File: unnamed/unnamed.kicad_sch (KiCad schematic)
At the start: 70 parts, among them J1 Serial, J2 Serial, SW1 SW_Push, SW10 SW_Push, SW11 SW_Push, SW12 SW_Push, SW13 SW_Push, SW14 SW_Push, SW15 SW_Push, SW16 SW_Push, SW17 SW_Push, SW18 SW_Push, SW19 SW_Push, SW2 SW_Push, SW20 SW_Push, SW21 SW_Push, SW22 SW_Push, SW23 SW_Push, SW24 SW_Push, SW25 SW_SPST, SW26 SW_SPST, SW3 SW_Push, SW4 SW_Push, SW5 SW_Push, SW6 SW_Push, SW7 SW_Push, SW8 SW_Push, SW9 SW_Push, U1 eliteC, U2 eliteC

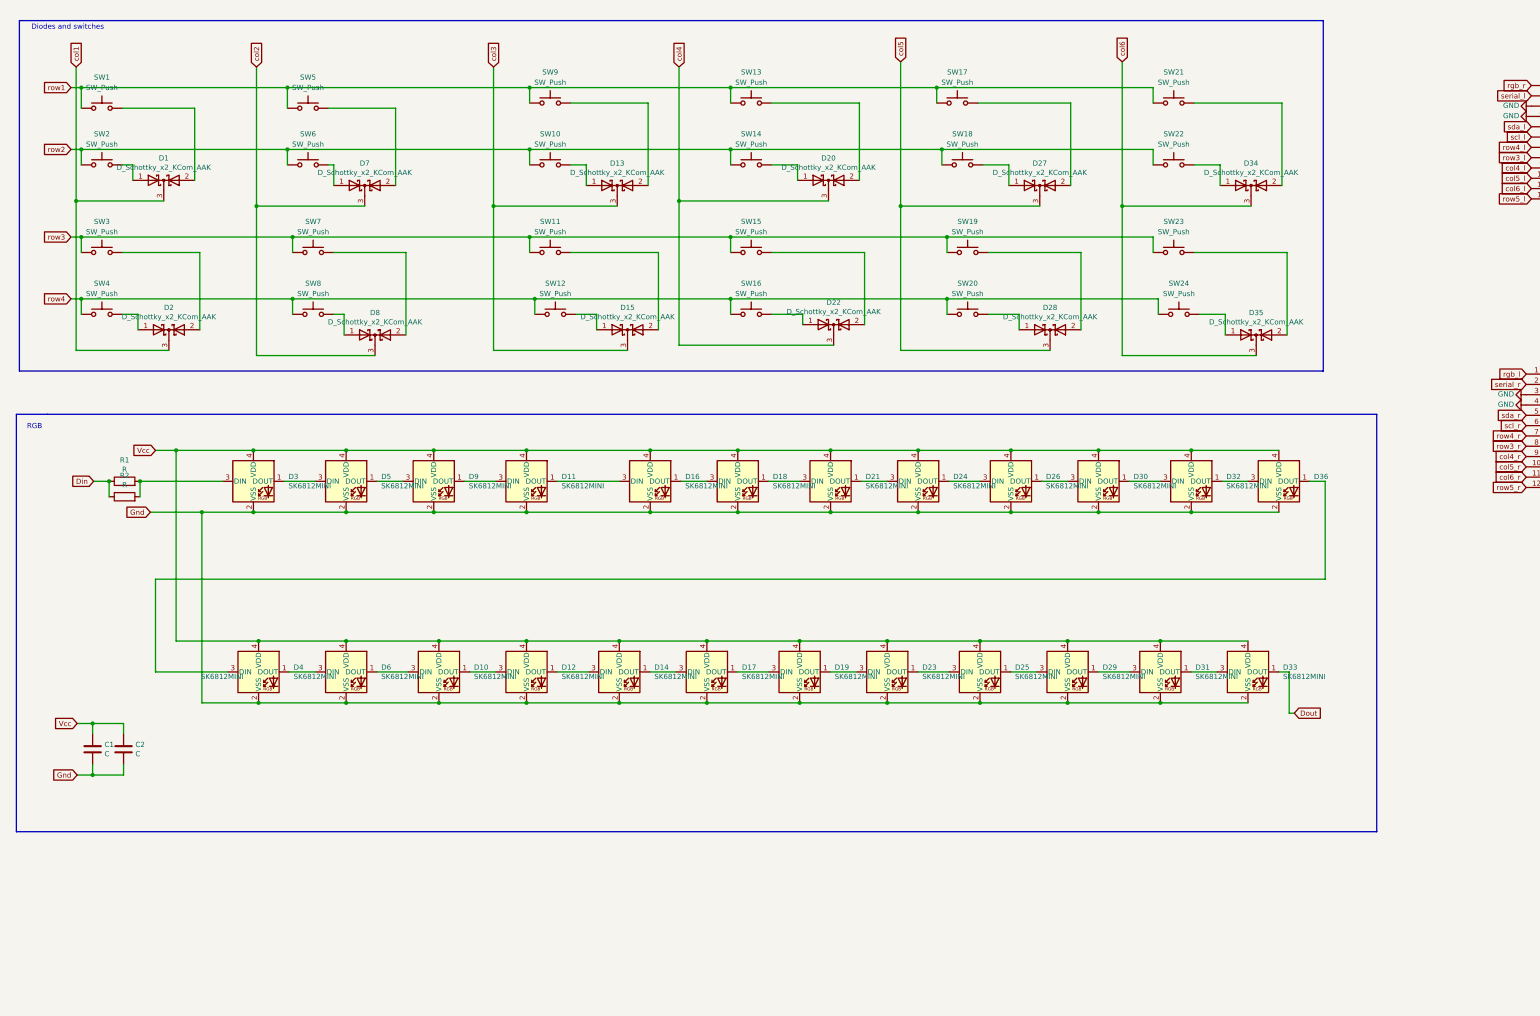
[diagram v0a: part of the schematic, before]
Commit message: go back to 3x5
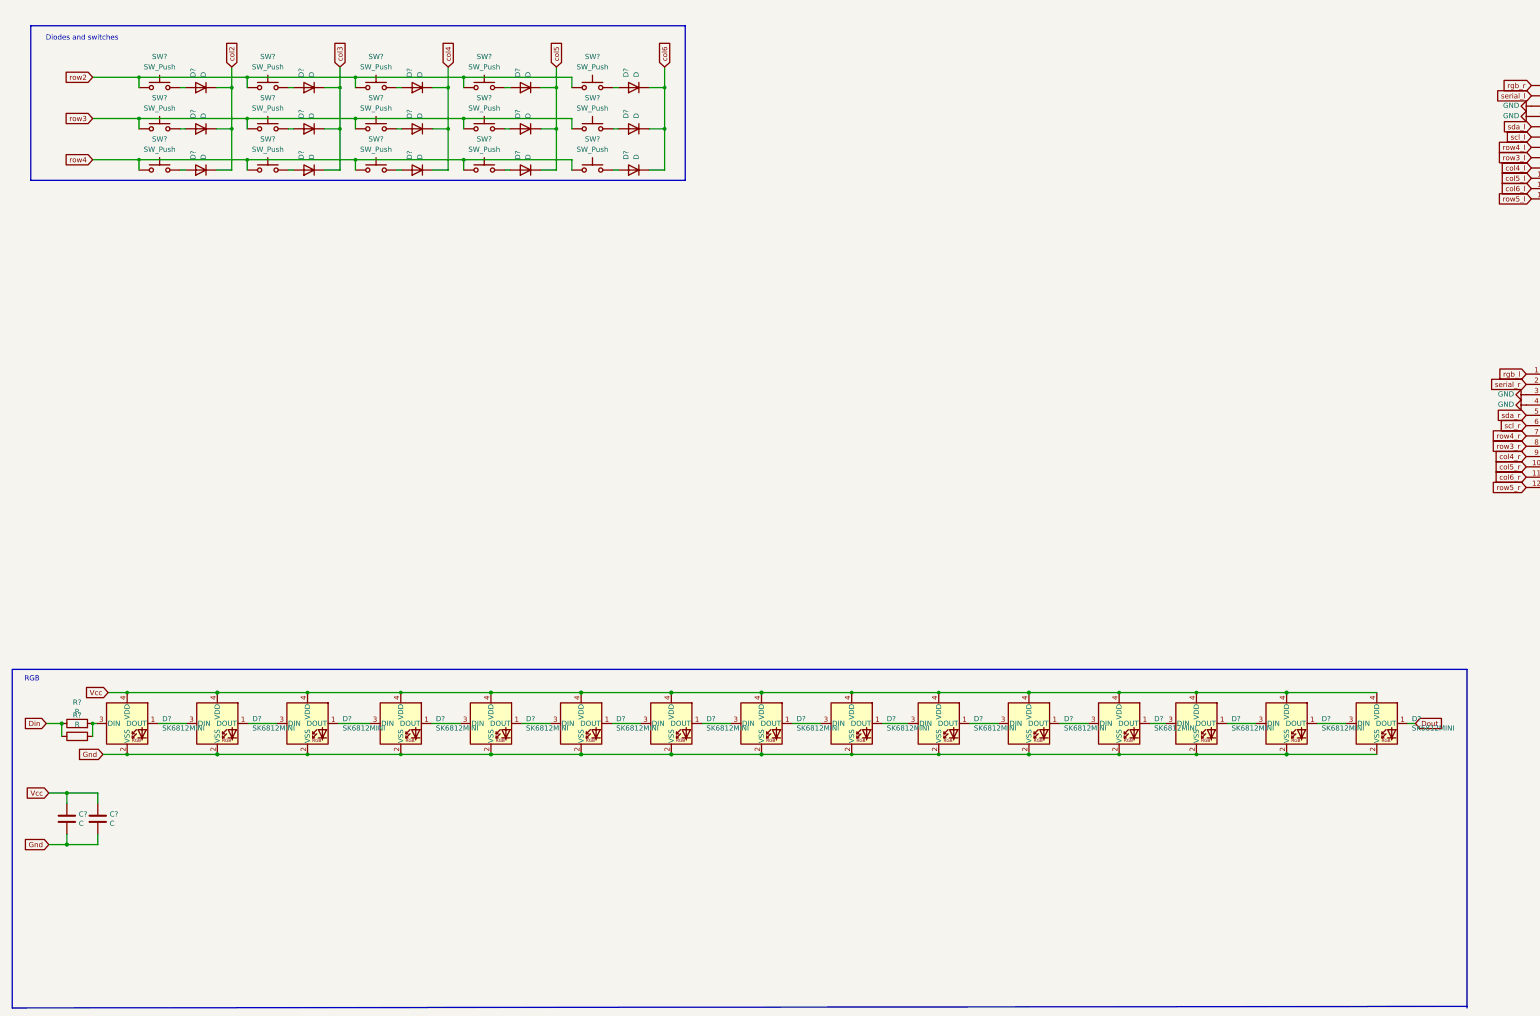
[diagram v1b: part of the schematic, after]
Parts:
- removed C1, C2: C, Capacitor_SMD:C_1206_3216Metric_Pad1.42x1.75mm_HandSolder, symbol Device:C
- removed D1, D13, D15, D2, D20, D22, D27, D28, D34, D35, D7, D8: D_Schottky_x2_KCom_AAK, customs:TSOT-23_HandSoldering, symbol Device:D_Schottky_x2_KCom_AAK
- removed D10, D11, D12, D14, D16, D17, D18, D19, D21, D23, D24, D25, D26, D29, D3, D30, D31, D32, D33, D36, D4, D5, D6, D9: SK6812MINI, libs2:YS-SK6812MINI-E_REVERSE, symbol LED:SK6812MINI
- removed R1, R2: R, Resistor_SMD:R_1206_3216Metric_Pad1.42x1.75mm_HandSolder, symbol Device:R
- removed SW1, SW10, SW11, SW12, SW13, SW14, SW15, SW16, SW17, SW18, SW19, SW2, SW20, SW21, SW22, SW23, SW24, SW3, SW4, SW5, SW6, SW7, SW8, SW9: SW_Push, custom:SW_MX_reversible, symbol Switch:SW_Push
- added C? (x2): C, Capacitor_SMD:C_1206_3216Metric_Pad1.42x1.75mm_HandSolder, symbol Device:C
- added D? (x15): D, custom:Diode_TH_SOD123, symbol Device:D
- added D? (x15): SK6812MINI, libs2:YS-SK6812MINI-E_REVERSE, symbol LED:SK6812MINI
- added R? (x2): R, Resistor_SMD:R_1206_3216Metric_Pad1.42x1.75mm_HandSolder, symbol Device:R
- added SW? (x15): SW_Push, custom:SW_MX_reversible, symbol Switch:SW_Push
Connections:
- net Din: now also R?.1, R?.1
- net Dout: now also D?.1 (DOUT)
- net Gnd: now also C?.2, C?.2, D?.2 (VSS), D?.2 (VSS), D?.2 (VSS), D?.2 (VSS), D?.2 (VSS), D?.2 (VSS), D?.2 (VSS), D?.2 (VSS), D?.2 (VSS), D?.2 (VSS), D?.2 (VSS), D?.2 (VSS), D?.2 (VSS), D?.2 (VSS), D?.2 (VSS)
- net Vcc: now also C?.1, C?.1, D?.4 (VDD), D?.4 (VDD), D?.4 (VDD), D?.4 (VDD), D?.4 (VDD), D?.4 (VDD), D?.4 (VDD), D?.4 (VDD), D?.4 (VDD), D?.4 (VDD), D?.4 (VDD), D?.4 (VDD), D?.4 (VDD), D?.4 (VDD), D?.4 (VDD)
- net col2: now also D?.1 (K), D?.1 (K), D?.1 (K)
- net col3: now also D?.1 (K), D?.1 (K), D?.1 (K)
- net col4: now also D?.1 (K), D?.1 (K), D?.1 (K)
- net col5: now also D?.1 (K), D?.1 (K), D?.1 (K)
- net col6: now also D?.1 (K), D?.1 (K), D?.1 (K)
- net row2: now also SW?.1, SW?.1, SW?.1, SW?.1, SW?.1
- net row3: now also SW?.1, SW?.1, SW?.1, SW?.1, SW?.1
- net row4: now also SW?.1, SW?.1, SW?.1, SW?.1, SW?.1
- new net: D?.2 (A), SW?.2 (x15)
- new net: D?.1 (DOUT), D?.3 (DIN) (x14)
- new net: D?.3 (DIN), R?.2, R?.2
